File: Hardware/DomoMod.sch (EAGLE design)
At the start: 46 parts, among them Q1 BSS138, Q2 BSS138, T1 MMBT2222A, U1 BD9251FV, U2 CCS811, U3 BME280, U4 PIR

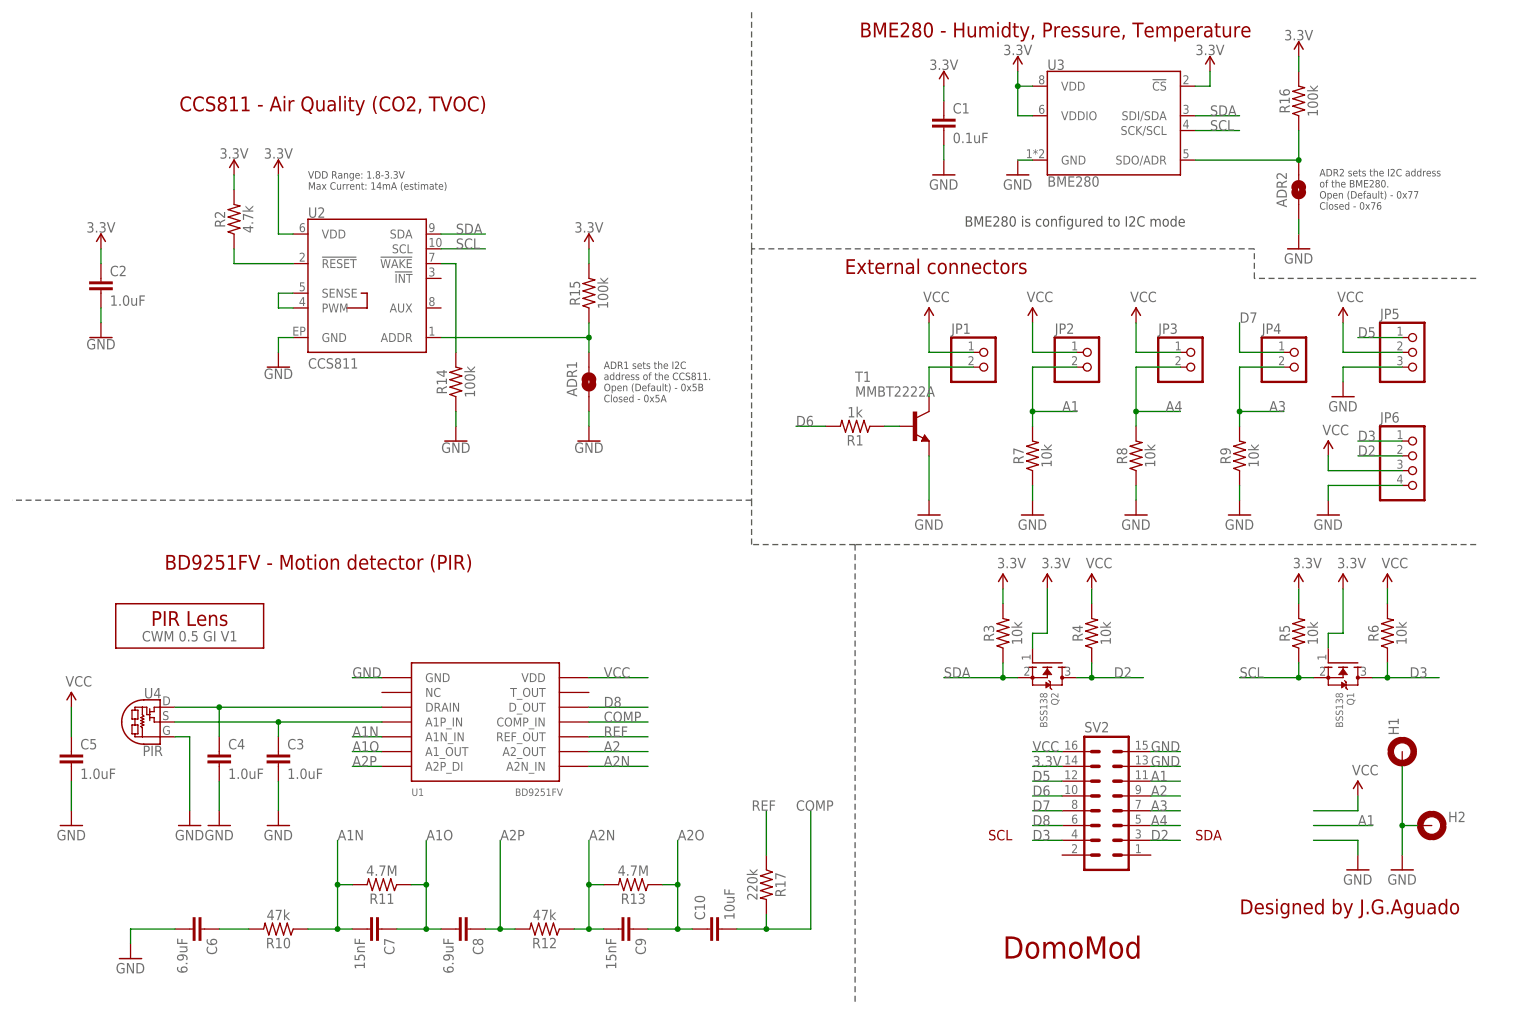
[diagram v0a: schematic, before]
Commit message: Updated design files
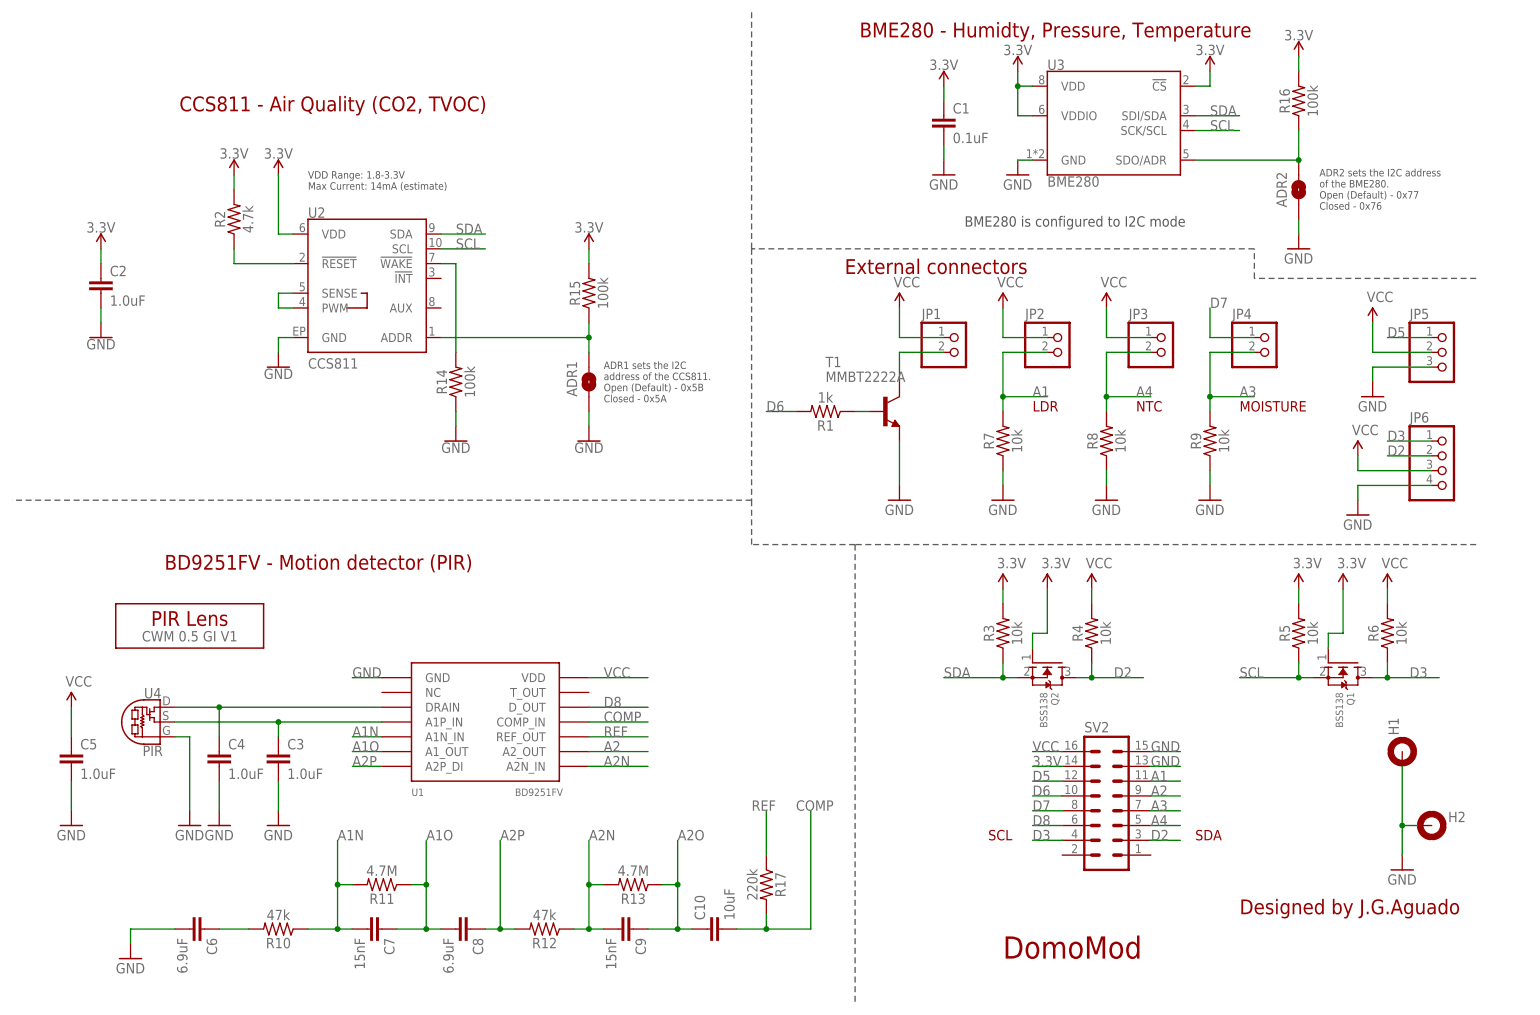
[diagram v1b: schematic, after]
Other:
- note added: "LDR"
- note added: "MOISTURE"
- note added: "NTC"
- moved on the sheet: JP1, JP2, JP3, JP4, JP5, JP6, R1, R7, R8, R9, T1
